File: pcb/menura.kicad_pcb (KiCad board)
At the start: 2 copper layers, 123 x 97.2 mm, 55 parts, among them SW1 SW_Push, SW10 SW_Push, SW11 SW_Push, SW12 SW_Push, SW13 SW_Push, SW14 SW_Push, SW15 SW_Push, SW16 SW_Push, SW17 SW_Push, SW18 SW_Push, SW19 SW_Push, SW2 SW_Push, SW20 SW_Push, SW21 SW_Push, SW22 SW_Push, SW3 SW_Push, SW4 SW_Push, SW5 SW_Push, SW6 SW_Push, SW7 SW_Push, SW8 SW_Push, SW9 SW_Push

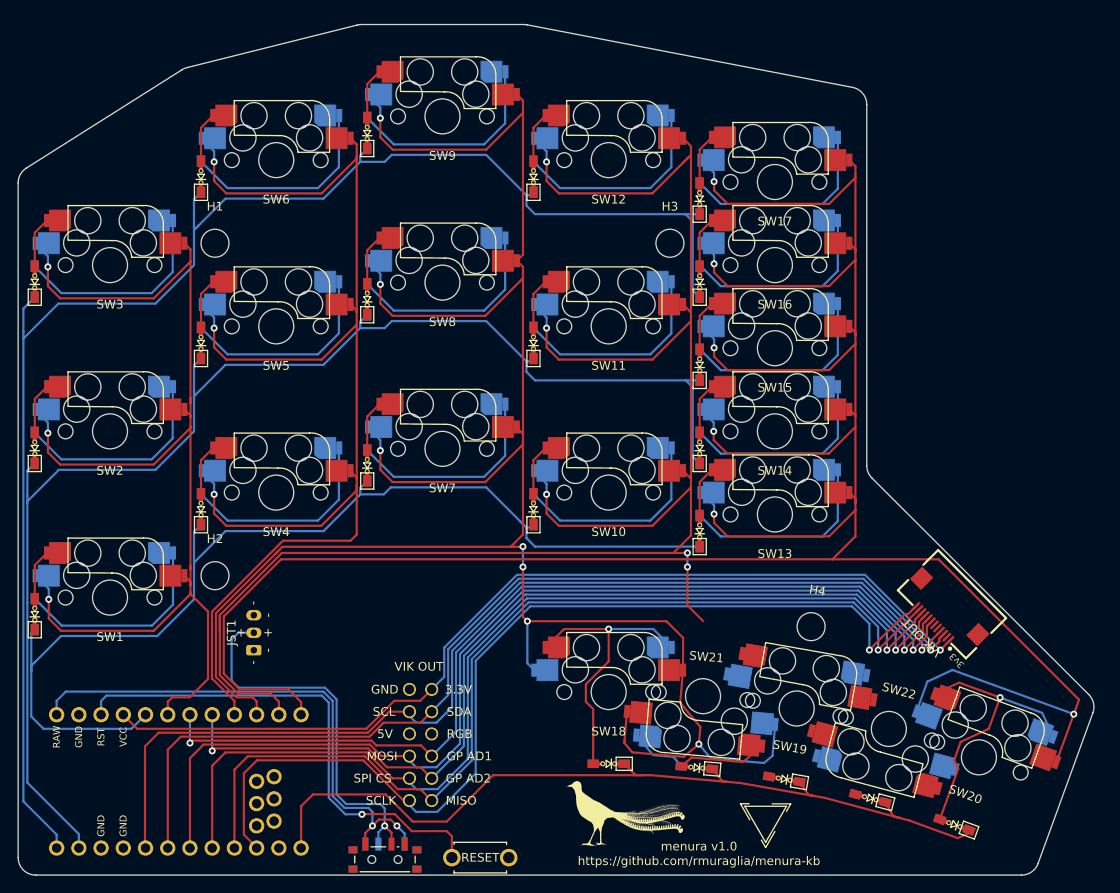
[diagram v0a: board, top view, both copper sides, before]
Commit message: thumbs sloppy but done
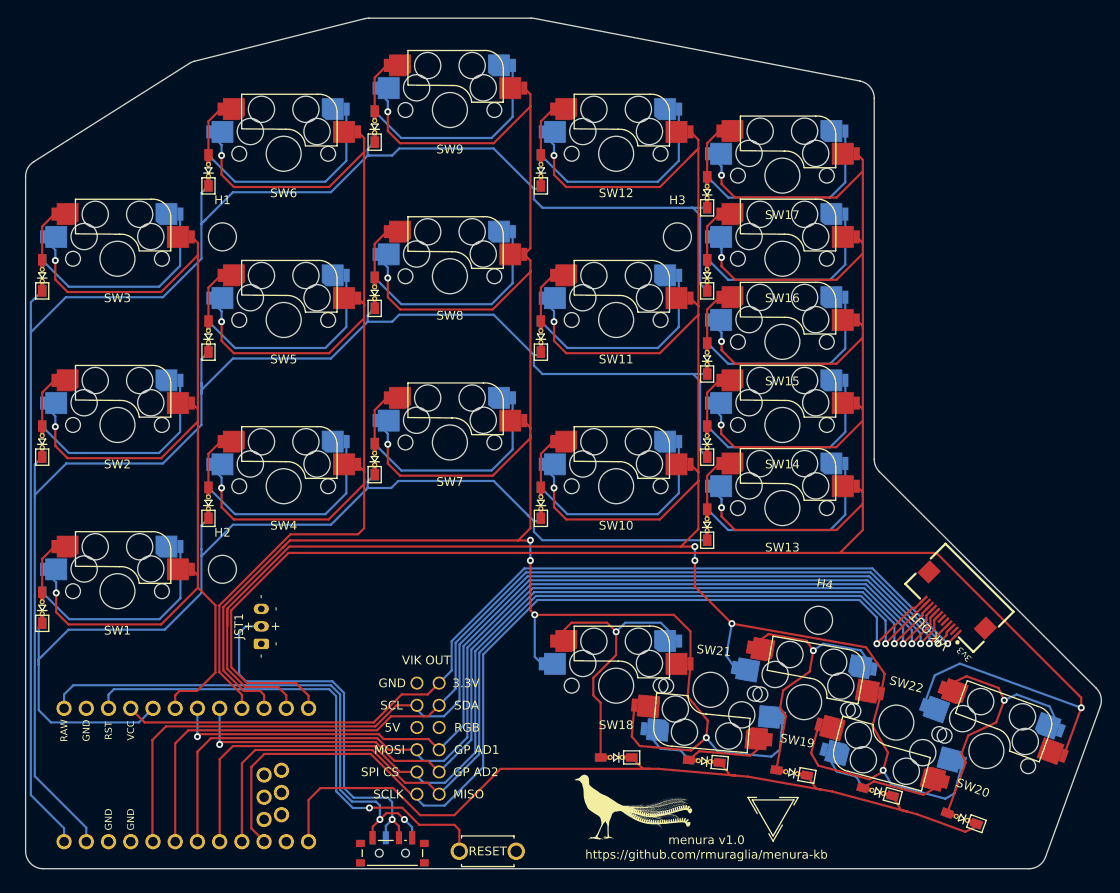
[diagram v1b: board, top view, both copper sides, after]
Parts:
- moved D14 1.12 mm to (168.9, 82.0)
- moved MCU1 1.12 mm to (108.5, 119.7)
- moved D10 1.12 mm to (149.9, 89.0)
- moved H3 1.12 mm to (165.5, 58.6)
- moved D17 1.12 mm to (168.9, 53.5)
- moved D6 1.12 mm to (111.9, 51.0)
- moved H1 1.12 mm to (113.5, 58.6)
- moved D7 1.12 mm to (130.9, 84.0)
- moved SW3 1.12 mm to (101.5, 61.1)
- moved SW21 1.12 mm to (169.2, 110.3)
- moved D8 1.12 mm to (130.9, 65.0)
- moved SW2 1.12 mm to (101.5, 80.1)
- moved SW4 1.12 mm to (120.5, 87.1)
- moved SW7 1.12 mm to (139.5, 82.1)
- moved D2 1.12 mm to (92.9, 82.0)
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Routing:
- net col3: track 208.7 -> 273.2 mm, vias 5 -> 7
- net Net-(D19-A): track 0.00 -> 32.3 mm, vias 0 -> 1
- net Net-(D22-A): track 0.00 -> 17.0 mm
- net col4: track 317.2 -> 316.2 mm
